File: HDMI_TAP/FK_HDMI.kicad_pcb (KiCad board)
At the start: 2 copper layers, 2 parts

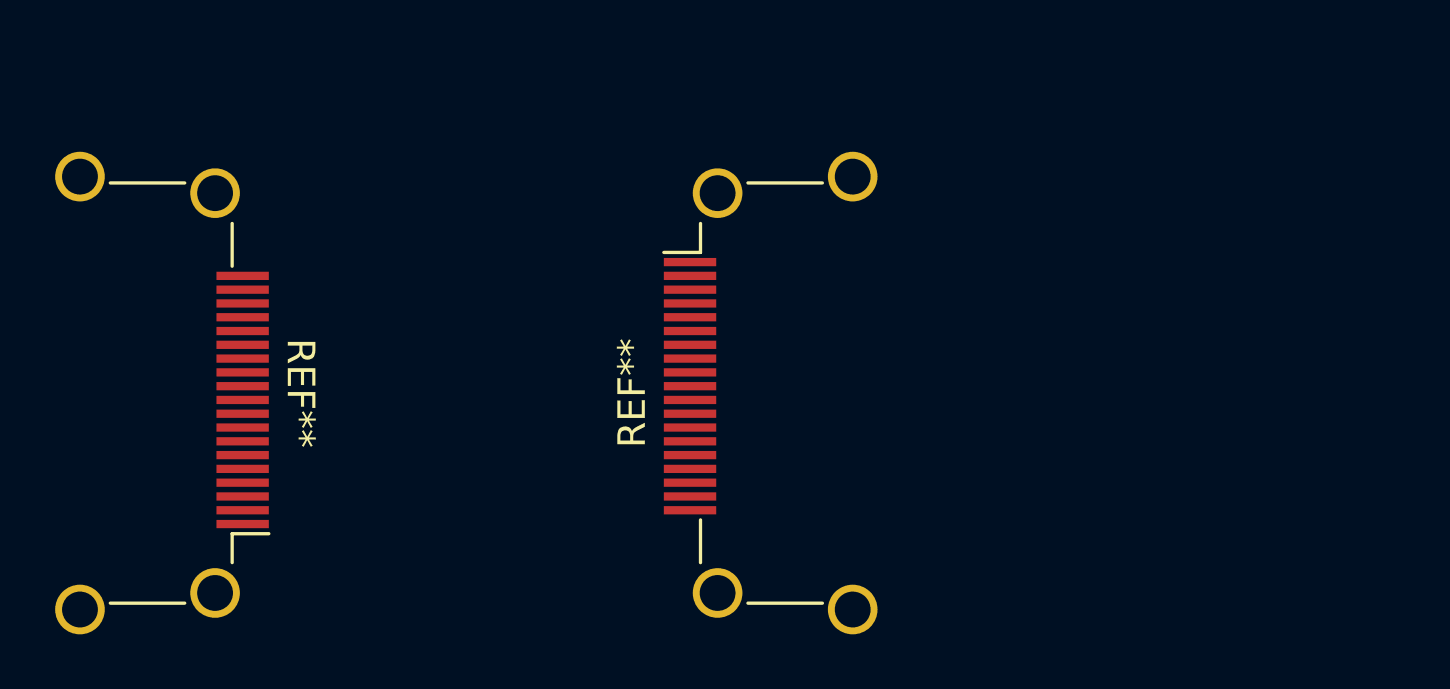
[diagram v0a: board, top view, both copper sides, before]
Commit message: Add files via upload
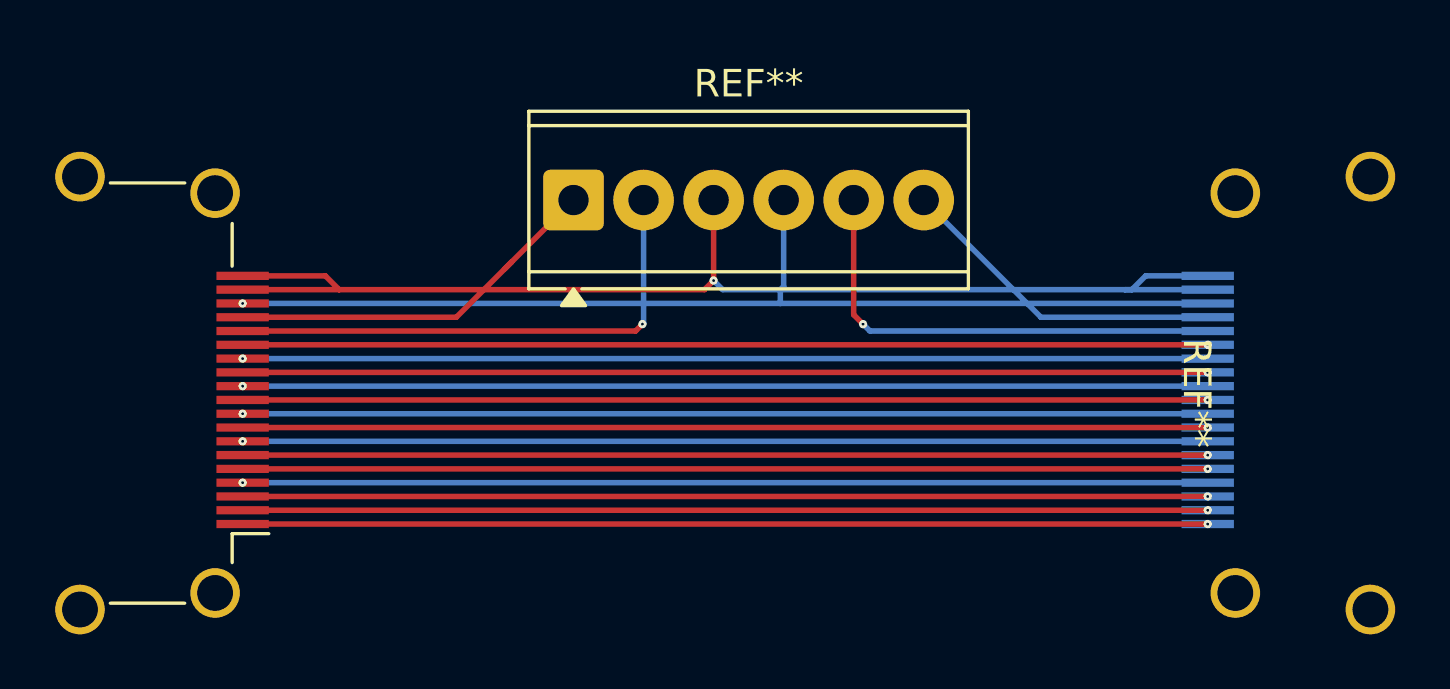
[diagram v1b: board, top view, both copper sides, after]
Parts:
- added REF**: TerminalBlock_Phoenix_MPT-0,5-6-2.54_1x06_P2.54mm_Horizontal, TerminalBlock_Phoenix:TerminalBlock_Phoenix_MPT-0,5-6-2.54_1x06_P2.54mm_Horizontal, F.Cu at (107.5, 80.0)
- REF**: moved to B.Cu
- moved REF** 18.8 mm to (135.5, 87.0), turned to -90 degrees
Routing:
- net (no net): track 0.00 -> 636.4 mm, vias 0 -> 21
